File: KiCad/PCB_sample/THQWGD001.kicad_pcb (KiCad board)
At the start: 2 copper layers, 65 x 30.9 mm, 35 parts, among them M1 MCU_XIAO-RP2040, SW1 Switch_Push

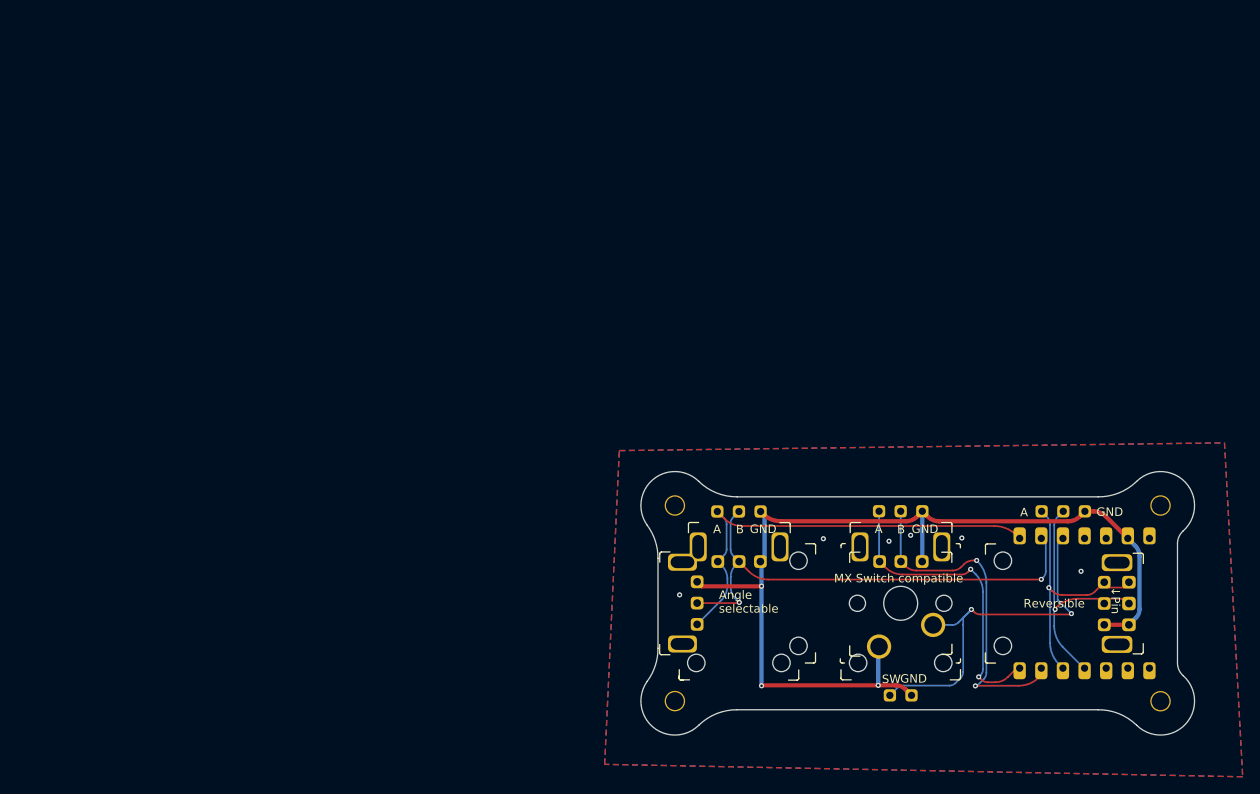
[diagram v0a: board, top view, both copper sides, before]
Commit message: 1.1
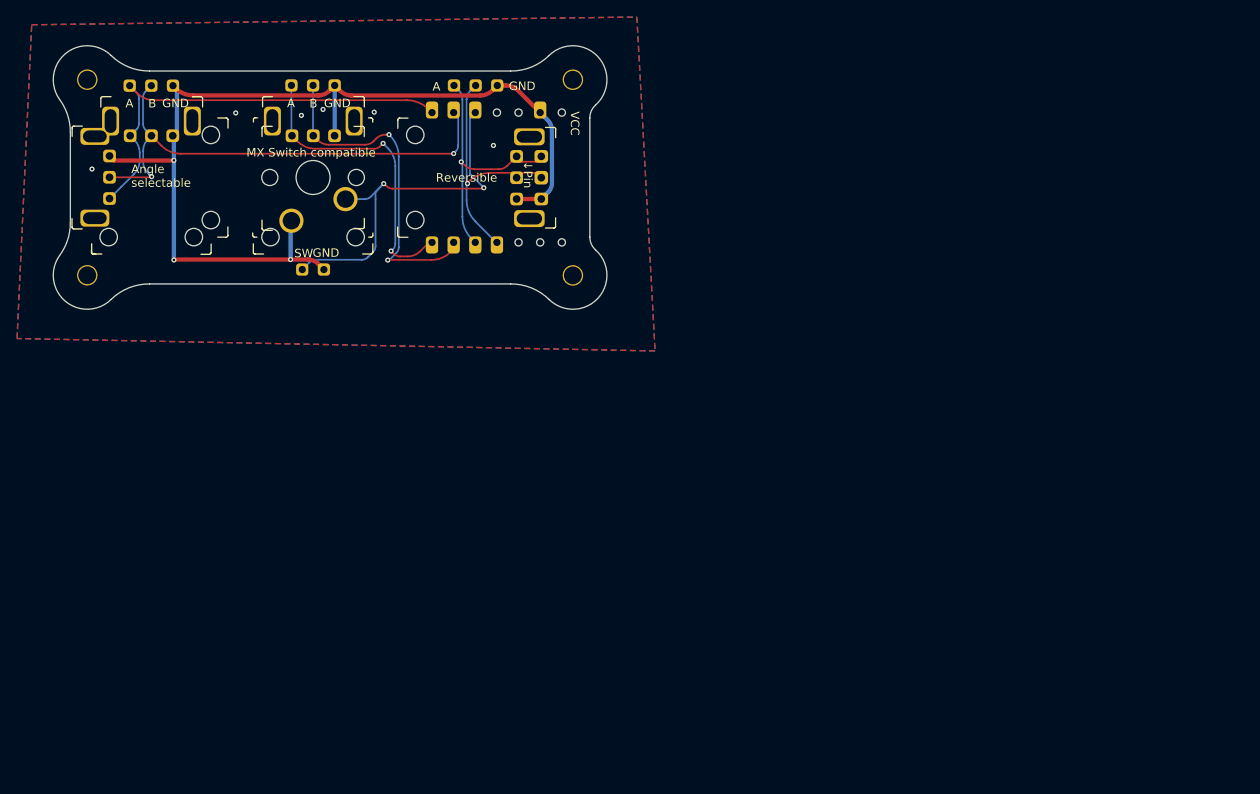
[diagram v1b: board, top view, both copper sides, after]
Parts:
- moved ? 85.2 mm to (-10.0, 5.81)
- moved ? 85.2 mm to (-11.2, -6.99)
- moved ? 85.2 mm to (-6.94, -6.95)
- moved ? 85.2 mm to (7.02, 7.79)
- moved ? 85.2 mm to (-27.1, 6.04)
- moved ? 85.2 mm to (-26.0, 8.95)
- moved ? 85.2 mm to (-24.8, 8.99)
- moved ? 85.2 mm to (-5.93, -8.29)
- moved ? 85.2 mm to (9.95, -5.77)
- moved ? 85.2 mm to (6.96, 6.95)
- moved ? 85.2 mm to (28.5, 4.74)
- moved ? 85.2 mm to (27.3, -5.88)
- moved ? 85.2 mm to (-28.3, -4.83)
- moved ? 85.2 mm to (-5.81, 8.99)
- moved ? 85.2 mm to (-12.0, 7.82)
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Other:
- board text added: "VCC"
